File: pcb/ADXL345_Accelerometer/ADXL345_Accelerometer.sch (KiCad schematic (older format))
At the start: 18 parts, among them J1 Conn_01x09, Q1 BSS138, Q2 BSS138, U1 ADXL345BCCZ, U2 AP2112K-3.3

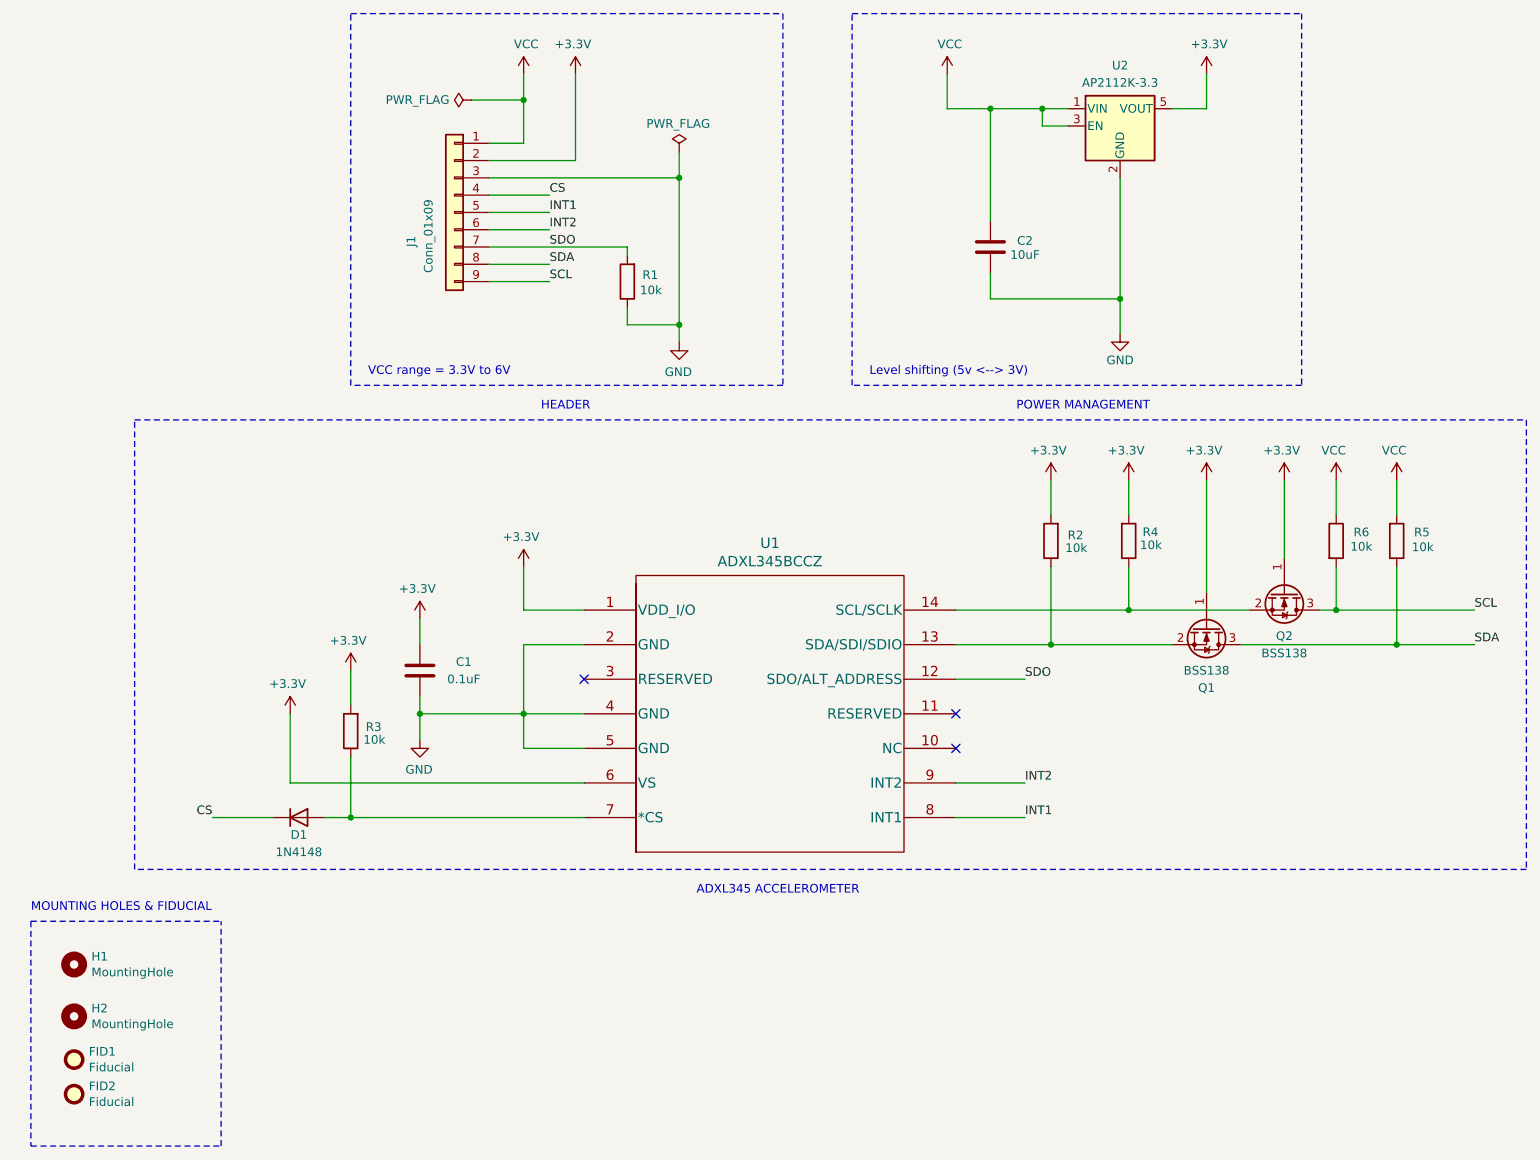
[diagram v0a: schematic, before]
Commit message: Modelos 3D
Se generaron los modelos 3D.
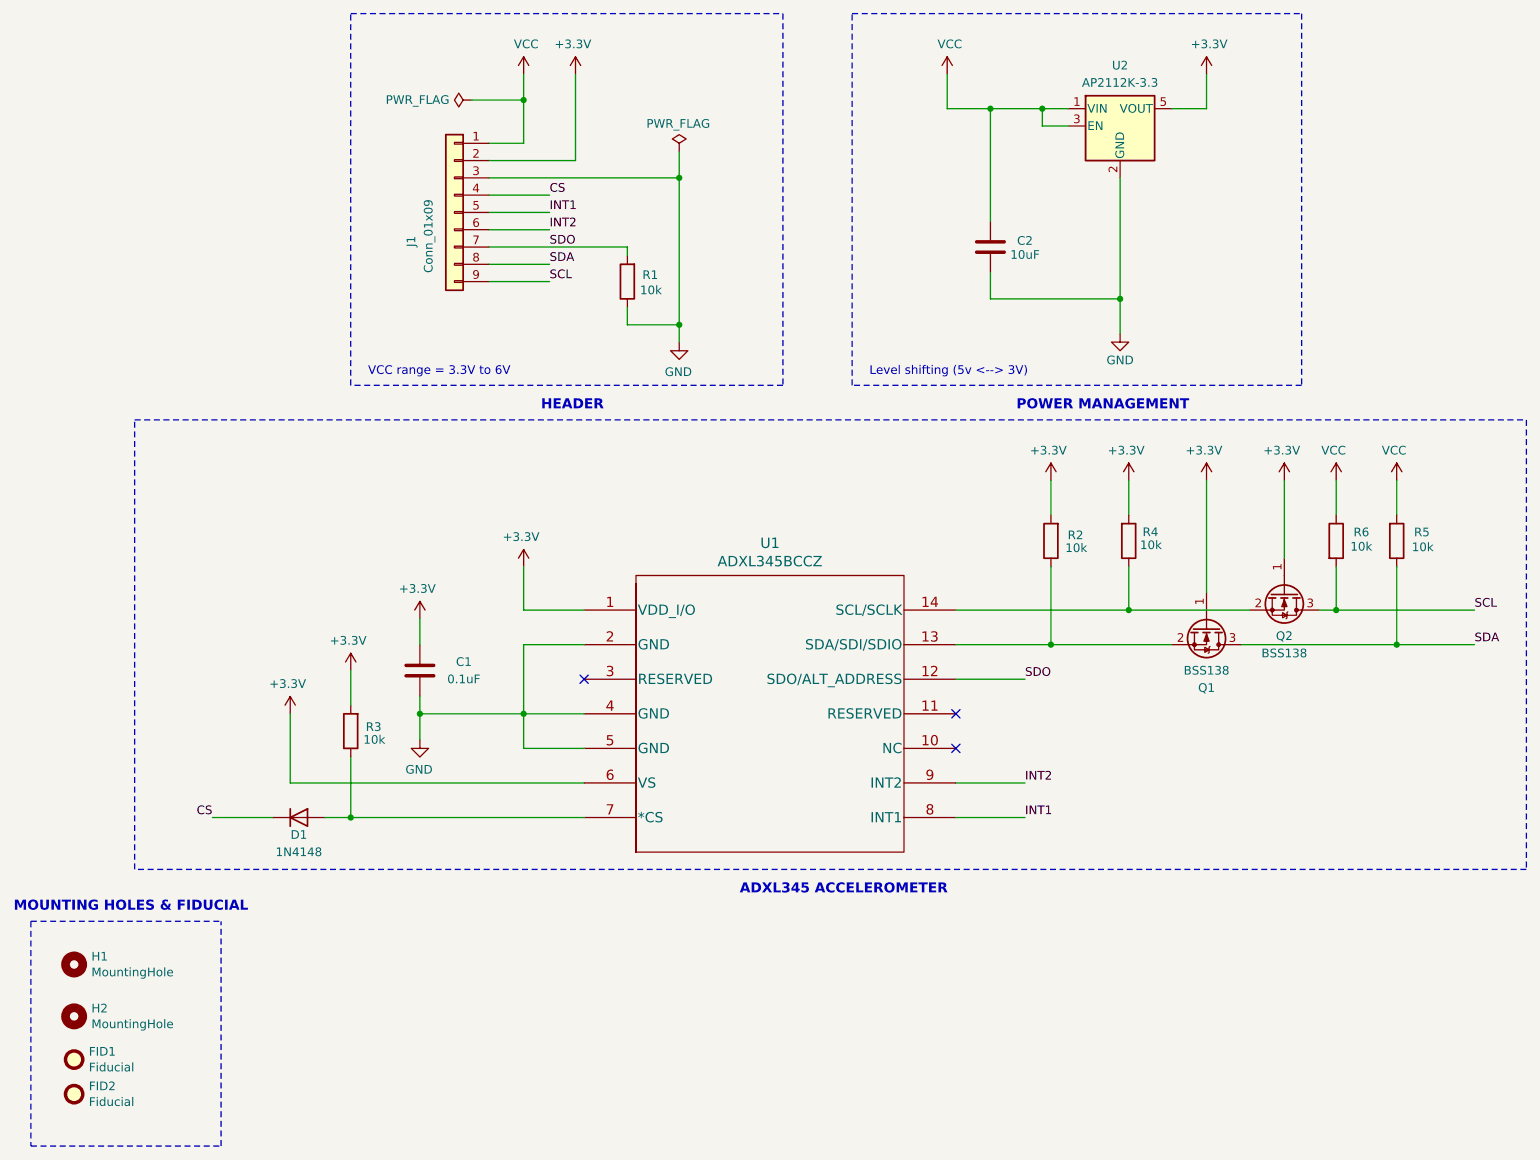
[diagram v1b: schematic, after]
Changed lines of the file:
@@
 	1    0    0    -1
 $EndComp
-Text Notes 1400 6050 0    50   ~ 0
+Text Notes 1300 6050 0    58   ~ 12
 MOUNTING HOLES & FIDUCIAL
 Wire Notes Line
@@
 	1    0    0    -1
 $EndComp
-Text Notes 5250 5950 0    50   ~ 0
+Text Notes 5500 5950 0    58   ~ 12
 ADXL345 ACCELEROMETER
 Text Notes 6250 2950 0    50   ~ 0
@@
 	1    0    0    -1
 $EndComp
-Text Notes 4350 3150 0    50   ~ 0
-HEADER
 Wire Notes Line
 	3250 850  5750 850
@@
 Wire Notes Line
 	8750 3000 6150 3000
-Text Notes 7100 3150 0    50   ~ 0
+Text Notes 7100 3150 0    58   ~ 12
 POWER MANAGEMENT
 $Comp
@@
 Wire Wire Line
 	9300 4500 9750 4500
+Text Notes 4350 3150 0    58   ~ 12
+HEADER
 $EndSCHEMATC
